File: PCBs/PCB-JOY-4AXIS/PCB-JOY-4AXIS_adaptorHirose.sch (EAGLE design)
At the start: 5 parts

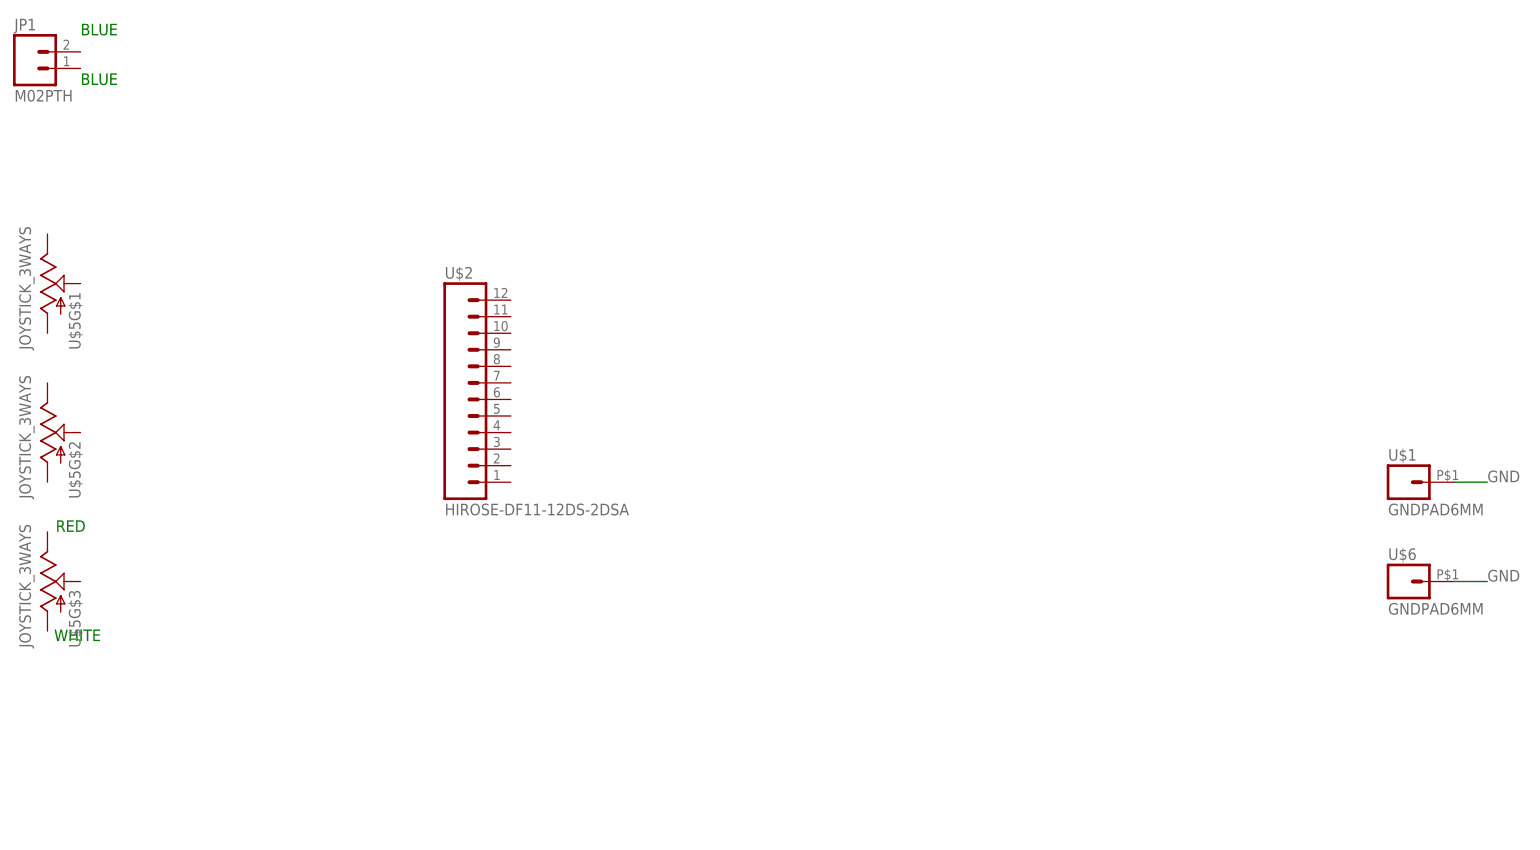
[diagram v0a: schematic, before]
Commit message: 4AXISHirose
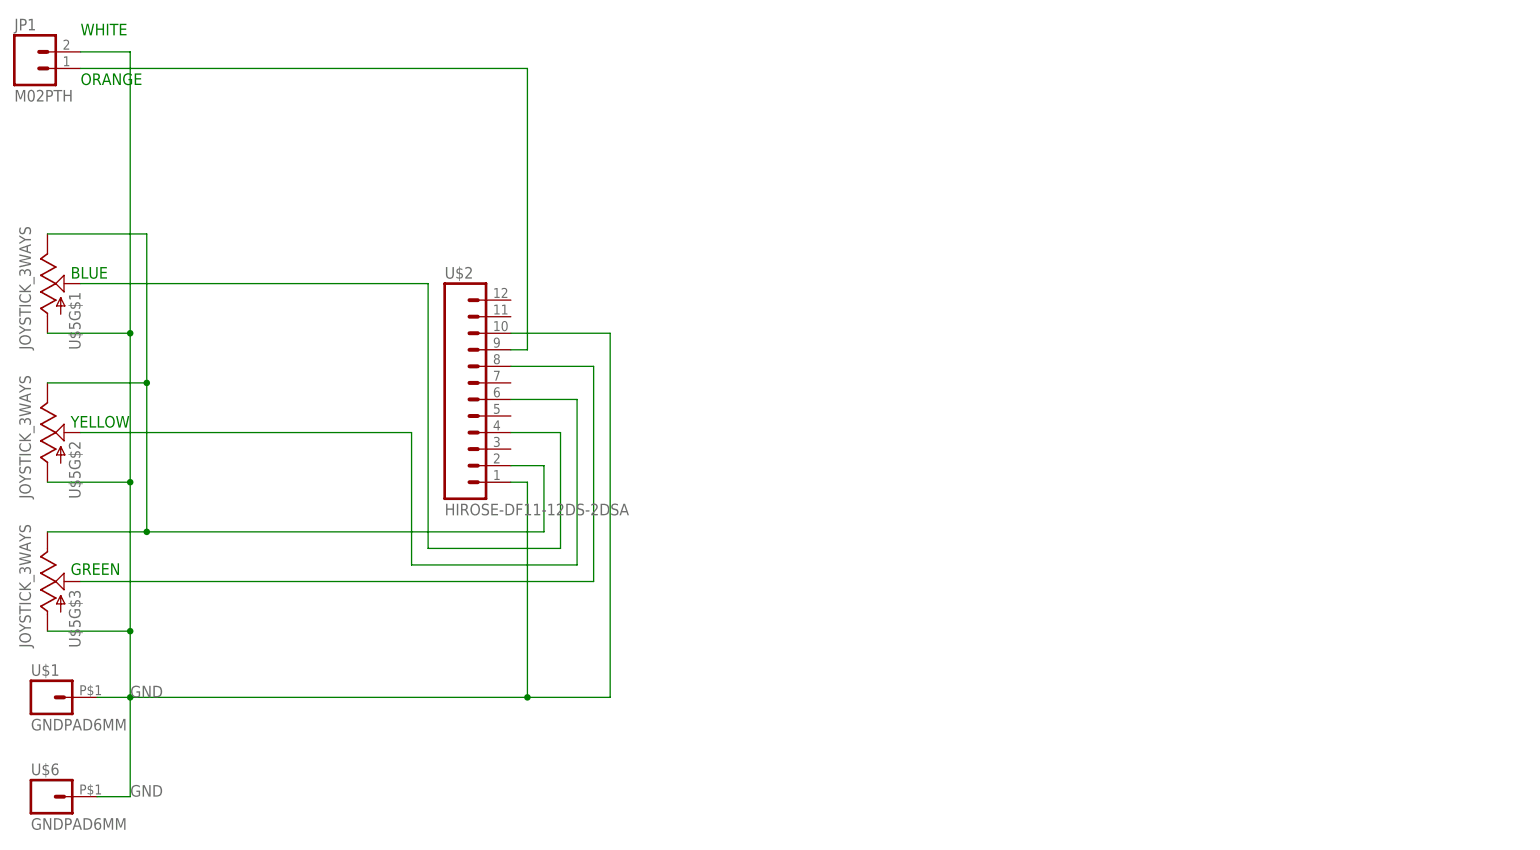
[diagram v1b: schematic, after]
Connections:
- new net N$1: U$2.2, U$5G$1.E, U$5G$2.E, U$5G$3.E
- new net N$2: U$2.4, U$5G$1.S
- new net N$3: U$2.6, U$5G$2.S
- new net N$4: U$2.8, U$5G$3.S
- new net N$5: JP1.1, U$2.9
- net GND: now also JP1.2, U$2.1, U$2.10, U$5G$1.A, U$5G$2.A, U$5G$3.A
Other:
- note added: "GREEN"
- note added: "ORANGE"
- note added: "YELLOW"
- note removed: "RED"
- moved on the sheet: U$1, U$6
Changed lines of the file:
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@@
 <sheet>
 <plain>
-<text x="-140.97" y="-15.24" size="1.778" layer="91">RED</text>
-<text x="-141.224" y="-32.004" size="1.778" layer="91">WHITE</text>
-<text x="-137.16" y="53.34" size="1.778" layer="91">BLUE</text>
-<text x="-137.16" y="60.96" size="1.778" layer="91">BLUE</text>
+<text x="-138.684" y="-21.844" size="1.778" layer="91">GREEN</text>
+<text x="-137.16" y="53.34" size="1.778" layer="91">ORANGE</text>
+<text x="-137.16" y="60.96" size="1.778" layer="91">WHITE</text>
+<text x="-138.684" y="0.762" size="1.778" layer="91">YELLOW</text>
+<text x="-138.684" y="23.622" size="1.778" layer="91">BLUE</text>
 </plain>
 <instances>
@@
 <instance part="U$5" gate="G$2" x="-142.24" y="0"/>
 <instance part="U$5" gate="G$3" x="-142.24" y="-22.86"/>
-<instance part="U$1" gate="G$1" x="68.58" y="-7.62"/>
-<instance part="U$6" gate="G$1" x="68.58" y="-22.86"/>
+<instance part="U$1" gate="G$1" x="-139.7" y="-40.64"/>
+<instance part="U$6" gate="G$1" x="-139.7" y="-55.88"/>
 <instance part="U$2" gate="G$1" x="-78.74" y="2.54"/>
 </instances>
@@
 <net name="GND" class="1">
 <segment>
+<pinref part="U$6" gate="G$1" pin="1"/>
+<wire x1="-134.62" y1="-55.88" x2="-129.54" y2="-55.88" width="0.1524" layer="91"/>
+<label x="-129.54" y="-55.88" size="1.778" layer="95"/>
 <pinref part="U$1" gate="G$1" pin="1"/>
-<wire x1="73.66" y1="-7.62" x2="78.74" y2="-7.62" width="0.1524" layer="91"/>
-<label x="78.74" y="-7.62" size="1.778" layer="95"/>
-</segment>
-<segment>
-<pinref part="U$6" gate="G$1" pin="1"/>
-<wire x1="73.66" y1="-22.86" x2="78.74" y2="-22.86" width="0.1524" layer="91"/>
-<label x="78.74" y="-22.86" size="1.778" layer="95"/>
+<wire x1="-134.62" y1="-40.64" x2="-129.54" y2="-40.64" width="0.1524" layer="91"/>
+<label x="-129.54" y="-40.64" size="1.778" layer="95"/>
+<pinref part="JP1" gate="G$1" pin="2"/>
+<wire x1="-137.16" y1="58.42" x2="-129.54" y2="58.42" width="0.1524" layer="91"/>
+<wire x1="-129.54" y1="58.42" x2="-129.54" y2="15.24" width="0.1524" layer="91"/>
+<pinref part="U$5" gate="G$1" pin="A"/>
+<wire x1="-129.54" y1="15.24" x2="-129.54" y2="-7.62" width="0.1524" layer="91"/>
+<wire x1="-129.54" y1="-7.62" x2="-129.54" y2="-30.48" width="0.1524" layer="91"/>
+<wire x1="-129.54" y1="-30.48" x2="-129.54" y2="-40.64" width="0.1524" layer="91"/>
+<wire x1="-142.24" y1="15.24" x2="-129.54" y2="15.24" width="0.1524" layer="91"/>
+<junction x="-129.54" y="15.24"/>
+<pinref part="U$5" gate="G$2" pin="A"/>
+<wire x1="-142.24" y1="-7.62" x2="-129.54" y2="-7.62" width="0.1524" layer="91"/>
+<junction x="-129.54" y="-7.62"/>
+<pinref part="U$5" gate="G$3" pin="A"/>
+<wire x1="-142.24" y1="-30.48" x2="-129.54" y2="-30.48" width="0.1524" layer="91"/>
+<junction x="-129.54" y="-30.48"/>
+<wire x1="-129.54" y1="-40.64" x2="-68.58" y2="-40.64" width="0.1524" layer="91"/>
+<wire x1="-68.58" y1="-40.64" x2="-68.58" y2="-7.62" width="0.1524" layer="91"/>
+<junction x="-129.54" y="-40.64"/>
+<pinref part="U$2" gate="G$1" pin="1"/>
+<wire x1="-68.58" y1="-7.62" x2="-71.12" y2="-7.62" width="0.1524" layer="91"/>
+<wire x1="-129.54" y1="-55.88" x2="-129.54" y2="-40.64" width="0.1524" layer="91"/>
+<pinref part="U$2" gate="G$1" pin="10"/>
+<wire x1="-71.12" y1="15.24" x2="-55.88" y2="15.24" width="0.1524" layer="91"/>
+<wire x1="-55.88" y1="15.24" x2="-55.88" y2="-40.64" width="0.1524" layer="91"/>
+<wire x1="-55.88" y1="-40.64" x2="-68.58" y2="-40.64" width="0.1524" layer="91"/>
+<junction x="-68.58" y="-40.64"/>
 </segment>
 </net>
+<net name="N$1" class="0">
+<segment>
+<pinref part="U$5" gate="G$3" pin="E"/>
+<wire x1="-142.24" y1="-15.24" x2="-127" y2="-15.24" width="0.1524" layer="91"/>
+<wire x1="-127" y1="-15.24" x2="-127" y2="7.62" width="0.1524" layer="91"/>
+<pinref part="U$5" gate="G$2" pin="E"/>
+<wire x1="-127" y1="7.62" x2="-142.24" y2="7.62" width="0.1524" layer="91"/>
+<pinref part="U$5" gate="G$1" pin="E"/>
+<wire x1="-142.24" y1="30.48" x2="-127" y2="30.48" width="0.1524" layer="91"/>
+<wire x1="-127" y1="30.48" x2="-127" y2="7.62" width="0.1524" layer="91"/>
+<junction x="-127" y="7.62"/>
+<wire x1="-127" y1="-15.24" x2="-66.04" y2="-15.24" width="0.1524" layer="91"/>
+<wire x1="-66.04" y1="-15.24" x2="-66.04" y2="-5.08" width="0.1524" layer="91"/>
+<junction x="-127" y="-15.24"/>
+<pinref part="U$2" gate="G$1" pin="2"/>
+<wire x1="-66.04" y1="-5.08" x2="-71.12" y2="-5.08" width="0.1524" layer="91"/>
+</segment>
+</net>
+<net name="N$2" class="0">
+<segment>
+<pinref part="U$5" gate="G$1" pin="S"/>
+<wire x1="-137.16" y1="22.86" x2="-83.82" y2="22.86" width="0.1524" layer="91"/>
+<wire x1="-83.82" y1="22.86" x2="-83.82" y2="-17.78" width="0.1524" layer="91"/>
+<wire x1="-83.82" y1="-17.78" x2="-63.5" y2="-17.78" width="0.1524" layer="91"/>
+<wire x1="-63.5" y1="-17.78" x2="-63.5" y2="0" width="0.1524" layer="91"/>
+<pinref part="U$2" gate="G$1" pin="4"/>
+<wire x1="-63.5" y1="0" x2="-71.12" y2="0" width="0.1524" layer="91"/>
+</segment>
+</net>
+<net name="N$3" class="0">
+<segment>
+<pinref part="U$5" gate="G$2" pin="S"/>
+<wire x1="-137.16" y1="0" x2="-86.36" y2="0" width="0.1524" layer="91"/>
+<wire x1="-86.36" y1="0" x2="-86.36" y2="-20.32" width="0.1524" layer="91"/>
+<wire x1="-86.36" y1="-20.32" x2="-60.96" y2="-20.32" width="0.1524" layer="91"/>
+<wire x1="-60.96" y1="-20.32" x2="-60.96" y2="5.08" width="0.1524" layer="91"/>
+<pinref part="U$2" gate="G$1" pin="6"/>
+<wire x1="-60.96" y1="5.08" x2="-71.12" y2="5.08" width="0.1524" layer="91"/>
+</segment>
+</net>
+<net name="N$4" class="0">
+<segment>
+<pinref part="U$5" gate="G$3" pin="S"/>
+<wire x1="-137.16" y1="-22.86" x2="-58.42" y2="-22.86" width="0.1524" layer="91"/>
+<wire x1="-58.42" y1="-22.86" x2="-58.42" y2="10.16" width="0.1524" layer="91"/>
+<pinref part="U$2" gate="G$1" pin="8"/>
+<wire x1="-58.42" y1="10.16" x2="-71.12" y2="10.16" width="0.1524" layer="91"/>
+</segment>
+</net>
+<net name="N$5" class="0">
+<segment>
+<pinref part="JP1" gate="G$1" pin="1"/>
+<wire x1="-137.16" y1="55.88" x2="-68.58" y2="55.88" width="0.1524" layer="91"/>
+<wire x1="-68.58" y1="55.88" x2="-68.58" y2="12.7" width="0.1524" layer="91"/>
+<pinref part="U$2" gate="G$1" pin="9"/>
+<wire x1="-68.58" y1="12.7" x2="-71.12" y2="12.7" width="0.1524" layer="91"/>
+</segment>
+</net>
